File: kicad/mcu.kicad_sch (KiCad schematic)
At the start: 3 parts

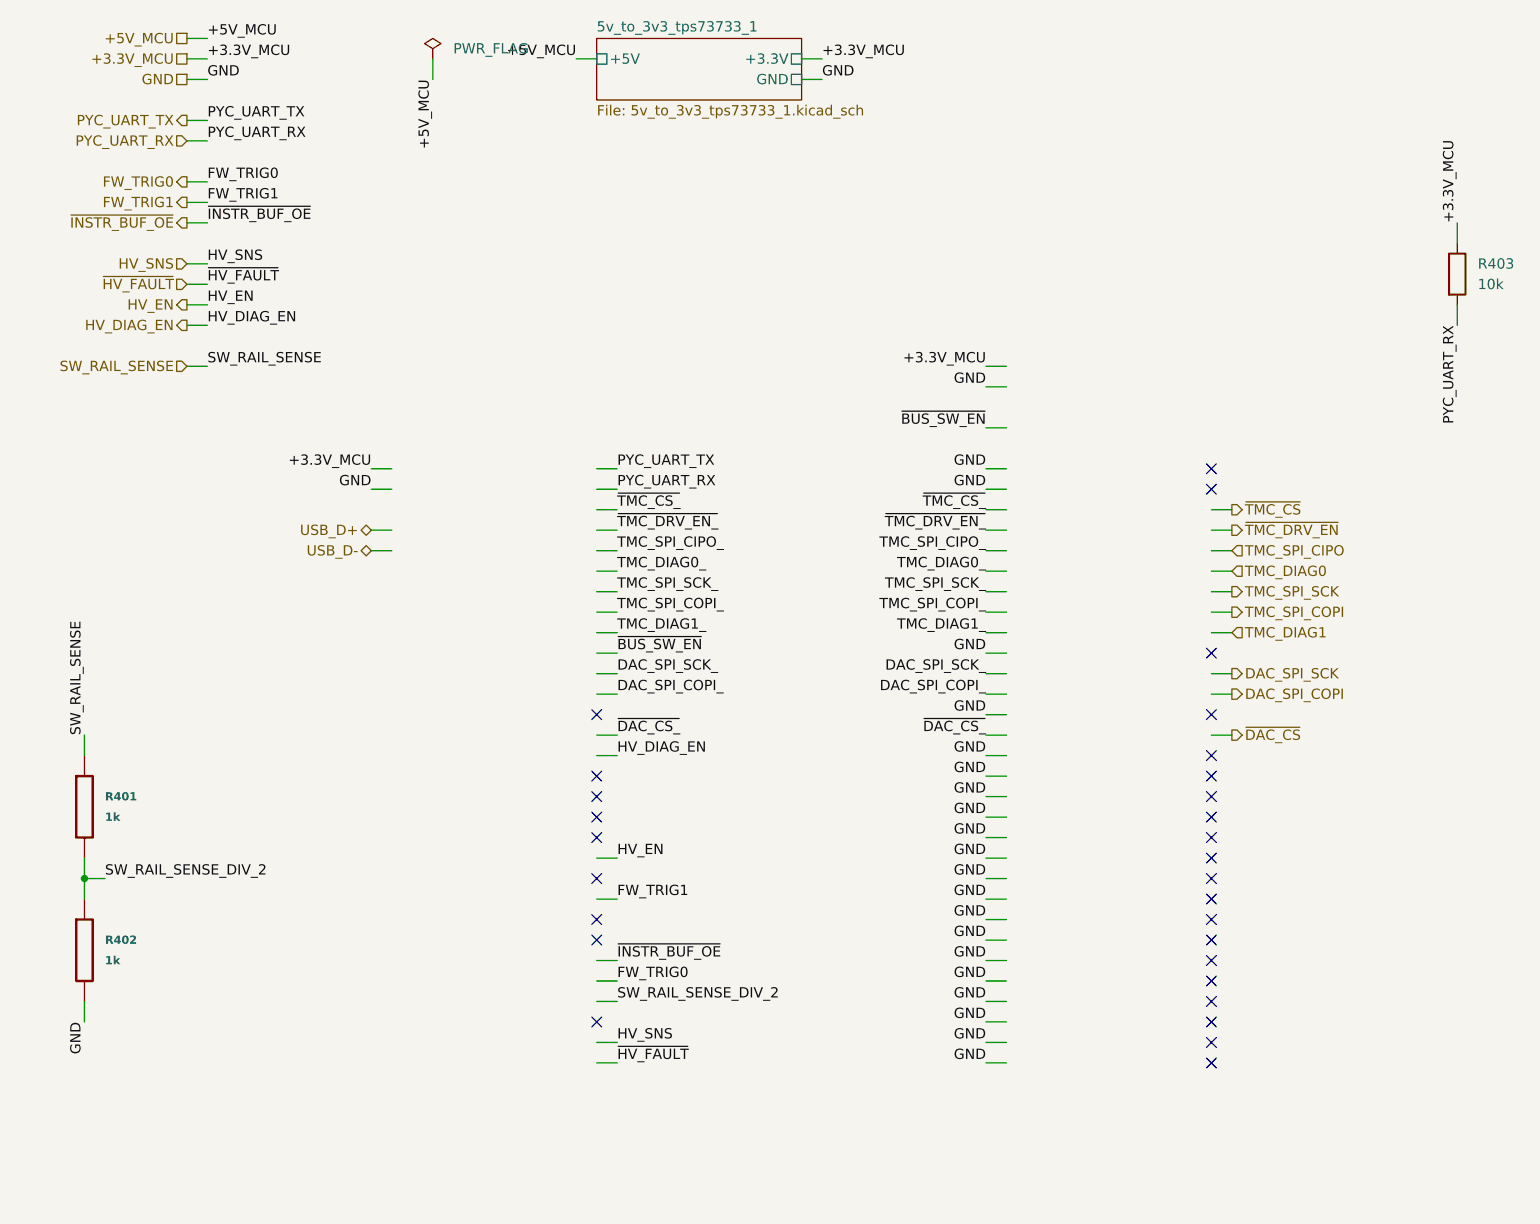
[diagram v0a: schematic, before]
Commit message: Progress towards v1.0
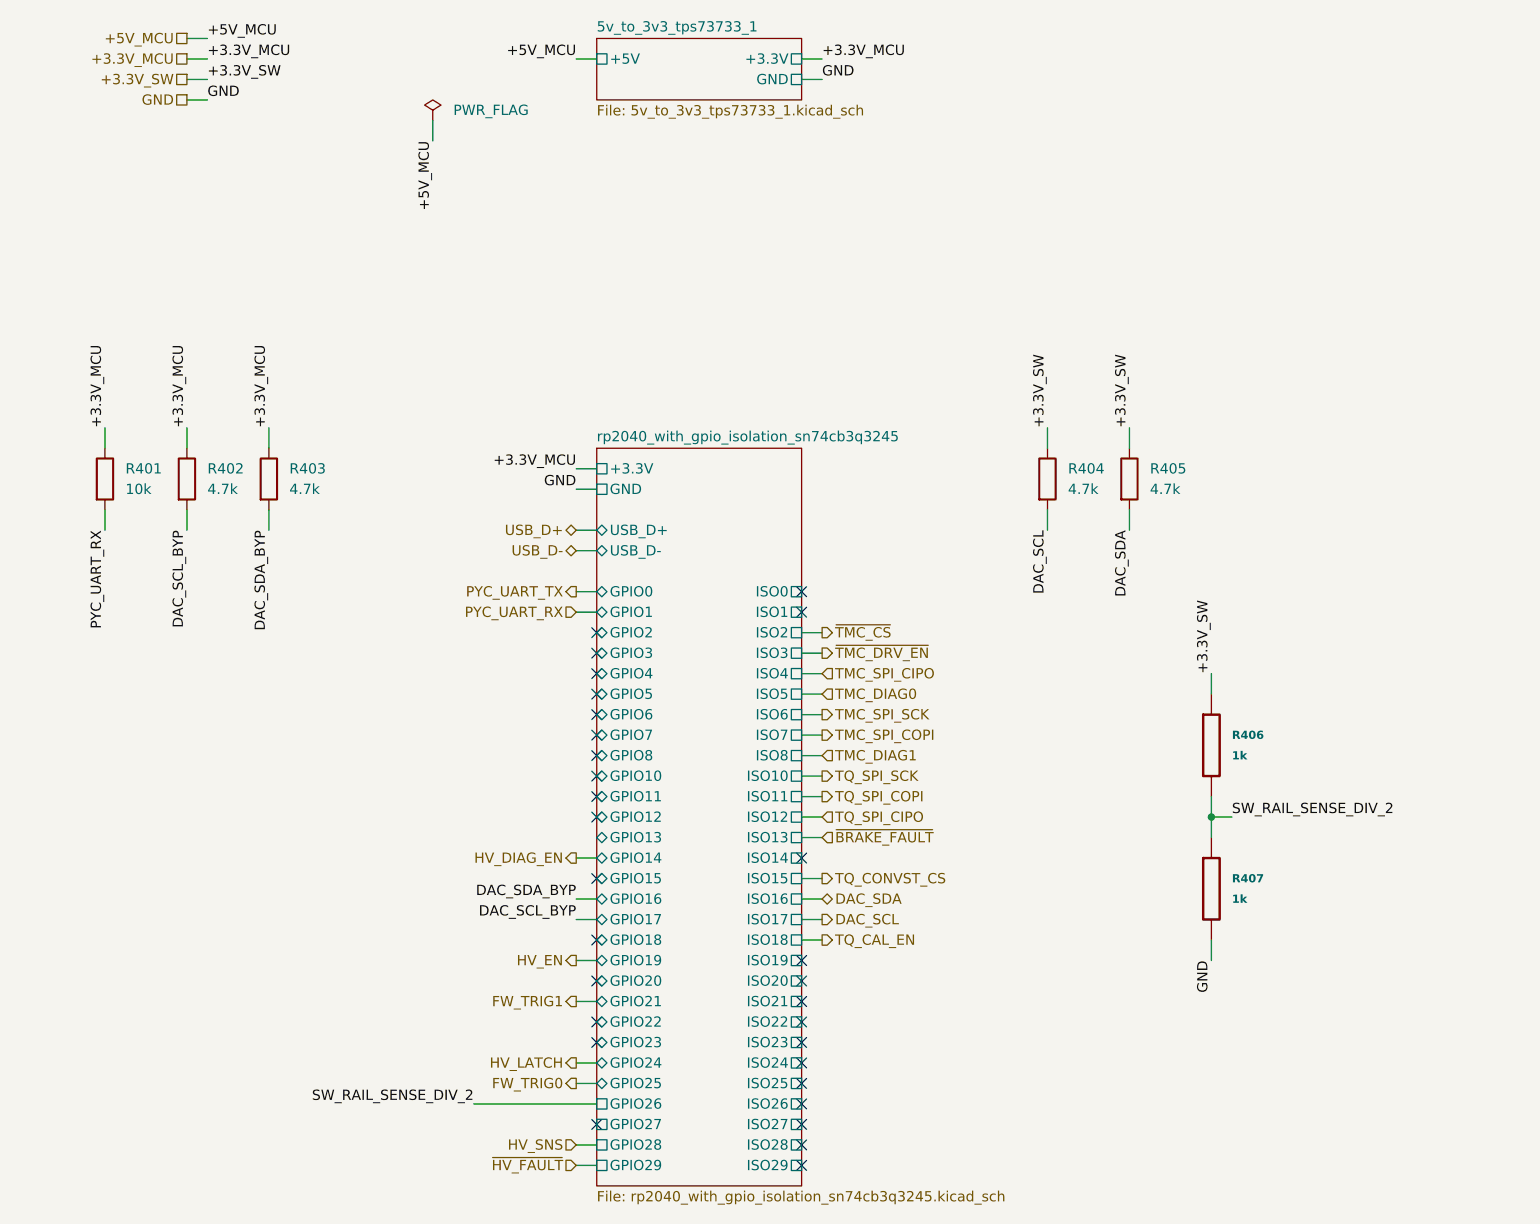
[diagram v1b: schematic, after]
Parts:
- added R402, R403, R404, R405: 4.7k, Resistor_SMD:R_0402_1005Metric, symbol orb_weaver_internal:All/OW-RES-4K7-0402
- renumbered R403 to R401, R401 to R406, R402 to R407
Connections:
- net +3.3V_MCU: now also R402.1, R403.1
- net SW_RAIL_SENSE renamed +3.3V_SW
- net +3.3V_SW: now also R404.1, R405.1
- new net DAC_SCL: R404.2
- new net DAC_SCL_BYP: R402.2
- new net DAC_SDA: R405.2
- new net DAC_SDA_BYP: R403.2
- no-connect marks 29 -> 30
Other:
- added sheet rp2040_with_gpio_isolation_sn74cb3q3245 (rp2040_with_gpio_isolation_sn74cb3q3245.kicad_sch)
- moved on the sheet: R401, R406, R407
